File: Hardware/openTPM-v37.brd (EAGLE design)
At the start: 45 x 19 mm, 67 parts, among them U1 SAM4S4A, U2 TPS62172, U3 TC58CVG0S3HQAIEWSON, Y1 12MHZ, Y2 32KHz

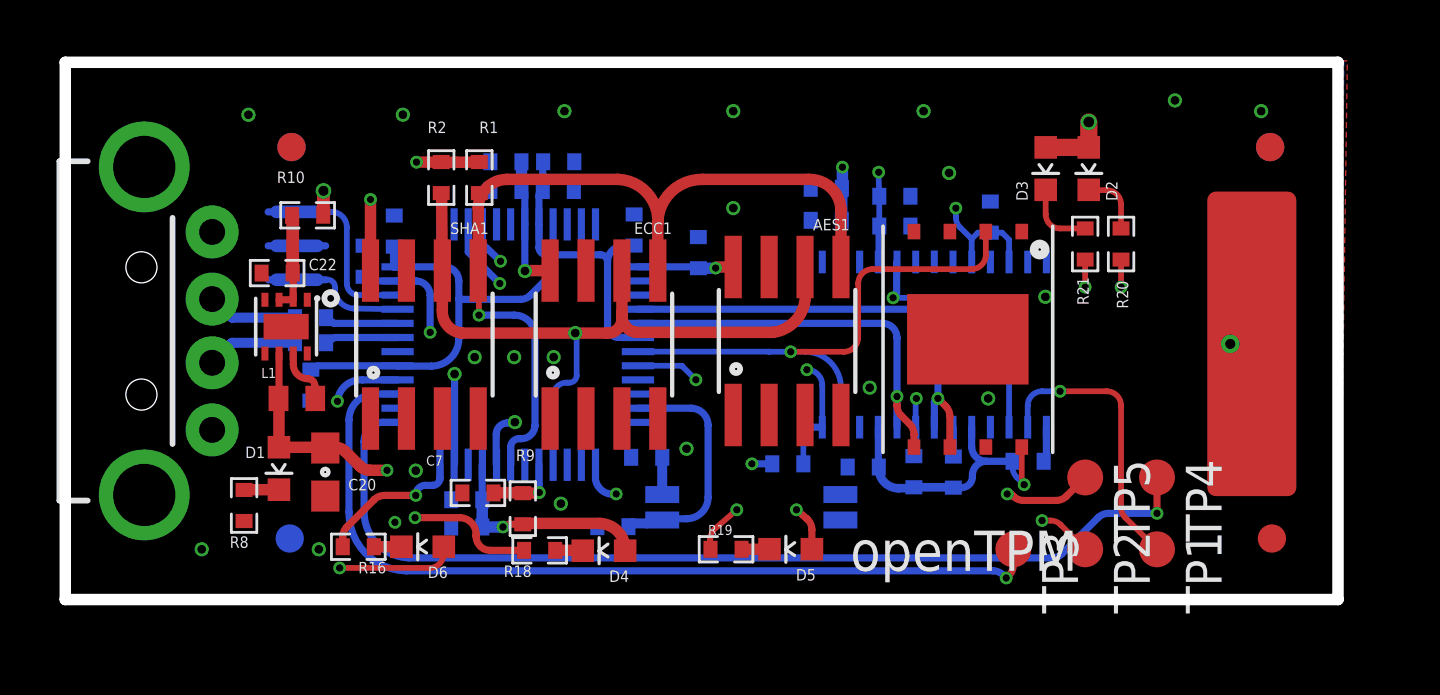
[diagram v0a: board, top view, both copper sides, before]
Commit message: OpenTPM v37 upload routing done
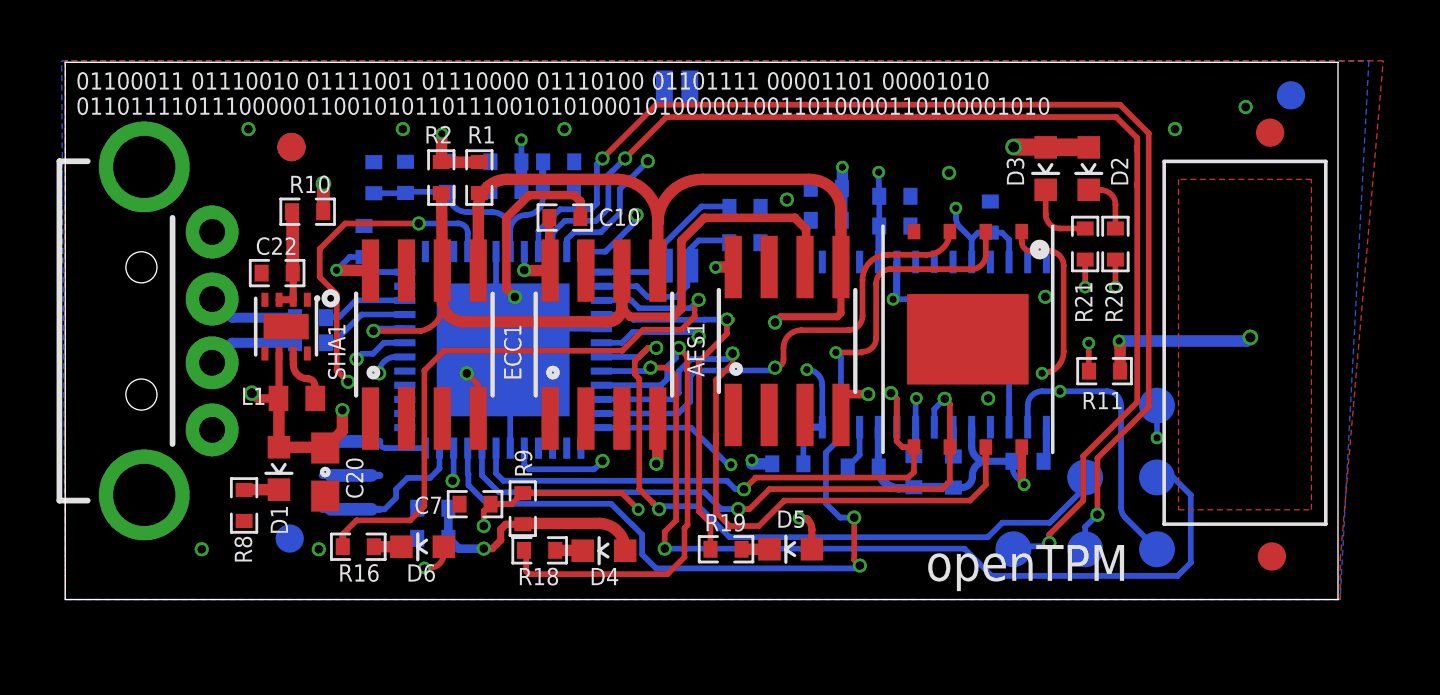
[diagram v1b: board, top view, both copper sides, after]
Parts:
- removed SL1: SLIDER_PASSIVE_1SEG, u2ftoken:SLIDER_PASSIVE_1SEG_12MM
- added 3V3: PTR1B1,27, CHEEPER-REV0.51A:B1,27
- added R11: 10K, TPM:0402
- U1: value SAM4S4A -> ATSAMD21G18_QFN; device TPM:LQFP-48 -> microbuilder:TQFN48_7MM
- moved C24 11.1 mm to (24.0, 12.6), turned to 180 degrees
- moved C23 9.50 mm to (24.0, 13.9), turned to 180 degrees
- moved Y1 8.34 mm to (10.1, 4.39), turned to 270 degrees
- moved C5 7.67 mm to (10.9, 14.9), turned to 90 degrees
- moved Y2 7.21 mm to (20.9, 11.2), turned to 90 degrees
- moved C18 6.87 mm to (13.5, 15.0)
- moved C10 4.88 mm to (17.7, 13.5), flipped to the top, turned to 0 degrees
- moved FID6 1.97 mm to (43.3, 17.8)
- moved C14 1.94 mm to (12.0, 14.9)
- moved C17 1.26 mm to (13.0, 2.17)
- moved C16 1.24 mm to (13.0, 3.23)
- moved C11 0.70 mm to (10.6, 12.7)
- moved FID3 0.63 mm to (42.7, 1.52)
- moved U1 0.55 mm to (15.5, 8.83), turned to 270 degrees
- moved FID1 0.51 mm to (42.6, 16.5)
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- renumbered TP1 to RST, TP2 to SWCLK, TP3 to SWDIO, TP4 to PB5, TP5 to PB4
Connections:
- removed net N$1: R4.2, U1.43
- removed net N$2: R3.2, U1.44
- removed net N$3: PB4.TP, U1.25
- removed net N$4: PB5.TP, U1.37
- removed net N$5: SWDIO.TP, U1.39
- removed net N$6: SWCLK.TP, U1.40
- new net CAP: R11.2
- new net DM: R4.2, U1.33
- new net DP: R3.2, U1.34
- new net N$19: U1.12, U3.1
- new net N$24: U1.10, U3.7
- new net N$25: U1.11, U3.3
- new net PB08: PB4.TP, U1.7
- new net PB09: PB5.TP, U1.8
- new net SLIDE: R11.1, U1.30
- new net SWCLK: SWCLK.TP, U1.45
- new net SWDIO: SWDIO.TP, U1.46
- net 1.2V: now also U1.43; no longer U1.18, U1.41, U1.48, U1.8
- net 3.3V: now also 3V3.TP, U1.17, U1.36, U1.44, U1.6; no longer U1.13, U1.33, U1.47, U1.7
- net AES: now also U1.4; no longer U1.35
- net CLK: now also U1.20; no longer U1.16
- net CS: now also U1.22; no longer U1.20
- net ECC: now also U1.9; no longer U1.32
- net GND: now also U1.18, U1.35, U1.42, U1.5, U1.THERMAL; no longer U1.2, U1.34
- net MISO: now also U1.21; no longer U1.19
- net MOSI: now also U1.19; no longer U1.17
- net N$8: now also U1.24; no longer U1.45
- net N$9: now also U1.23; no longer U1.46
- net RST: now also U1.40; no longer U1.29
- net SCL: now also U1.32; no longer U1.28
- net SHA: now also U1.3; no longer U1.36
- net STAT0: now also U1.47; no longer U1.3
- net STAT1: now also U1.48; no longer U1.4
- net XIN32: now also U1.1; no longer U1.24
- net XOUT32: now also U1.2; no longer U1.23
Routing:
- net SWDIO: track 0.00 -> 41.3 mm, vias 0 -> 2
- net SWCLK: track 0.00 -> 41.0 mm, vias 0 -> 2
- net N$6: track 34.6 -> 0.00 mm, vias 2 -> 0
- net N$4: track 34.5 -> 0.00 mm, vias 1 -> 0
- net PB09: track 0.00 -> 32.1 mm, vias 0 -> 2
- net N$5: track 30.6 -> 0.00 mm, vias 1 -> 0
- net SLIDE: track 0.00 -> 28.6 mm, vias 0 -> 2
- net GND: track 0.00 -> 26.1 mm, vias 21 -> 15
- net PB08: track 0.00 -> 25.3 mm, vias 0 -> 2
- net N$19: track 0.00 -> 25.0 mm, vias 0 -> 2
- net N$24: track 0.00 -> 24.1 mm, vias 0 -> 1
- net RST: track 35.2 -> 55.8 mm, vias 2 -> 5
- net N$3: track 18.4 -> 0.00 mm, vias 2 -> 0
- net SHA: track 5.41 -> 23.4 mm
- net N$25: track 0.00 -> 16.5 mm, vias 0 -> 1
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- added copper zone on layer 1, net CAP
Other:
- board text added: "01100011 01110010 01111001 01110000 01110100 01101111 00001101 00001010"
- board text added: "01101111 01110000 01100101 01101110 01010100 01010000 01001101 00001101 00001010"
- board text added: "011011110111000001100101011011100101010001010000010011010000110100001010"
